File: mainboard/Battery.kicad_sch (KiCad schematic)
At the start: 24 parts, among them IC602 USBLC6-2P6, IC701 BQ21040DBV, IC703 MAX17048, Q701 PMV50XNEAR, X701 USB, X702 Battery

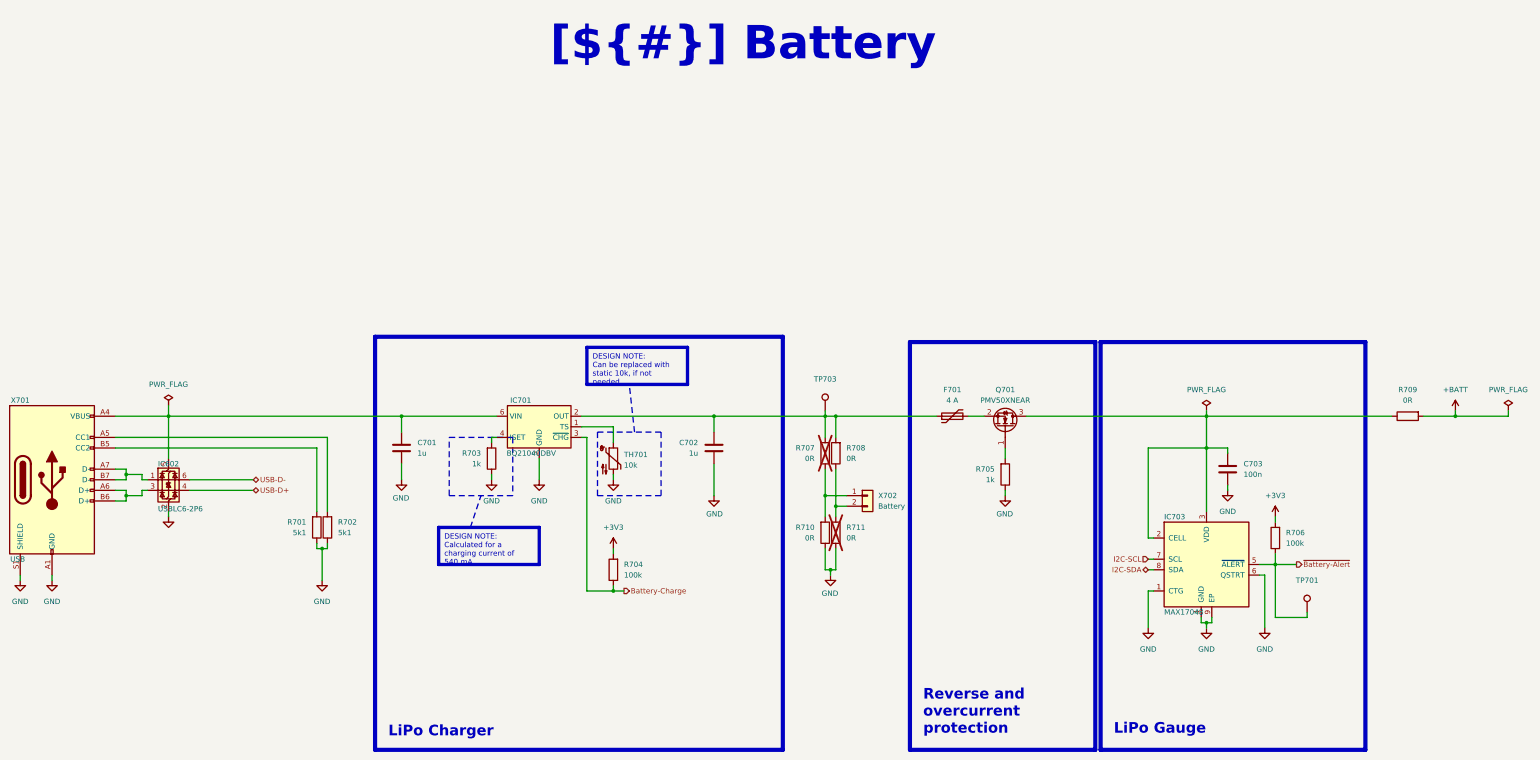
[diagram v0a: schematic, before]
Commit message: Layout complete
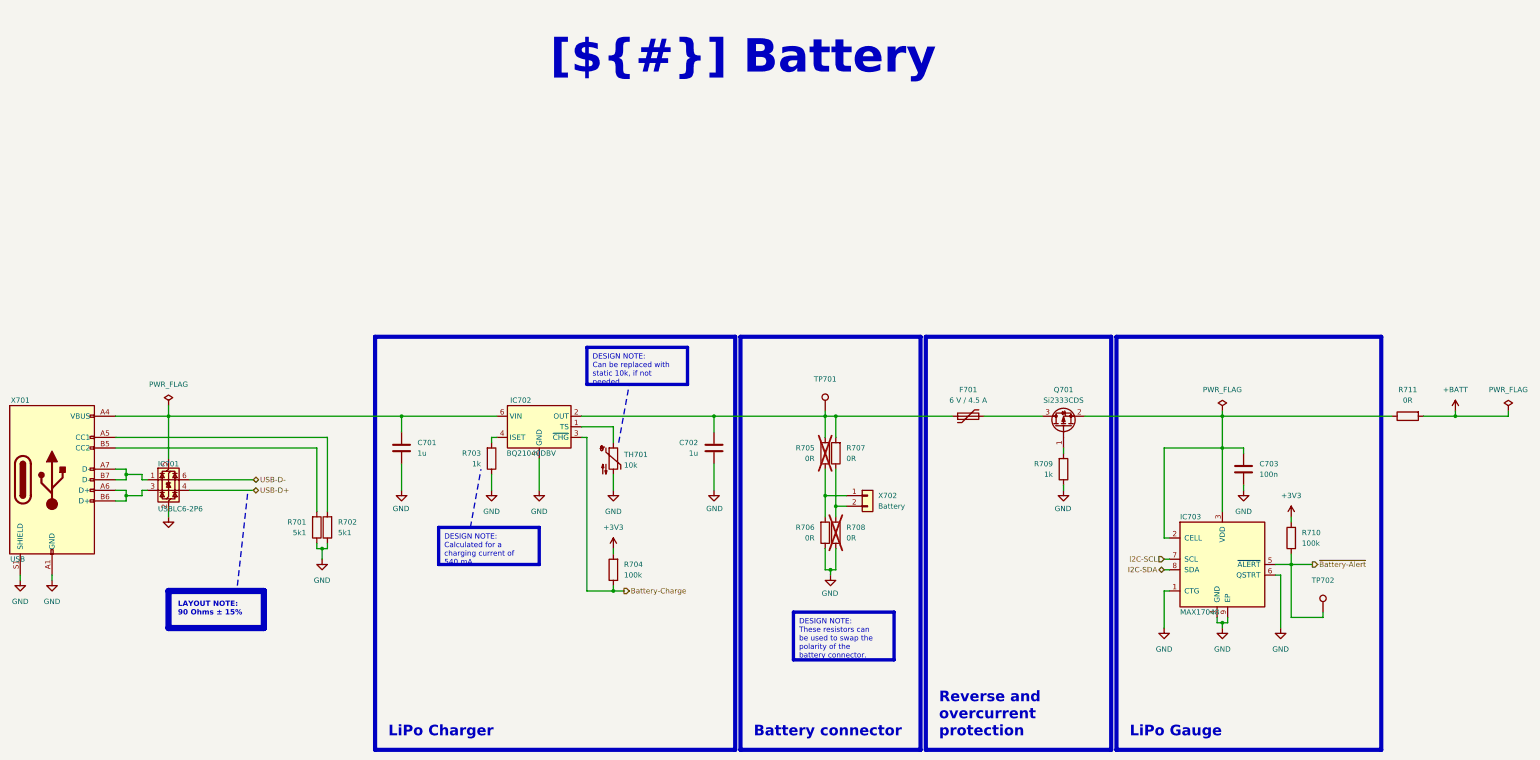
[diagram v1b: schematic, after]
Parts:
- F701: value 4 A -> 6 V / 4.5 A; manf# 1206L400SLWR -> 1206L450SLWR; mouser# 576-1206L400SLWR -> 576-1206L450SLWR
- Q701: value PMV50XNEAR -> Si2333CDS; footprint Package_TO_SOT_SMD:SOT-23 -> Package_TO_SOT_SMD:SOT-23-3; symbol Nexperia:PMV50XNEAR -> Vishay:Si2333CDS; manf Nexperia -> Vishay / Siliconix; manf# PMV50XNEAR -> SI2333CDS-T1-BE3; mouser# 771-PMV50XNEAR -> 78-SI2333CDS-T1-BE3
- X702: footprint Connector_JST:JST_PH_B2B-PH-SM4-TB_1x02-1MP_P2.00mm_Vertical -> JST:S2B-PH-SM4-TB; manf# B2B-PH-SM4-TB(LF)(SN) -> S2B-PH-SM4-TB(LF)(SN); mouser# 306-B2BPHSM4TBLFSN -> 306-S2B-PH-SM4-TB(LF)(SN)
- renumbered IC602 to IC701, IC701 to IC702, R707 to R705, R710 to R706, R708 to R707, R711 to R708, R705 to R709, R706 to R710, R709 to R711, TP703 to TP701, TP701 to TP702
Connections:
- net at Q701.2 (S): now also C703.1, IC703.2 (CELL), IC703.3 (VDD), R711.1; no longer F701.2
- new net: F701.2, Q701.3 (D)
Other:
- moved on the sheet: C703, F701, IC703, Q701, R709, R710, TP702
